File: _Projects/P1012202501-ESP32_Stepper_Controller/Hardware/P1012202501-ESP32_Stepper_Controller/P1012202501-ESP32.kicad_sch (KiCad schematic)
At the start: 6 parts, among them IC3 ESP32-WROOM-32UE-N16

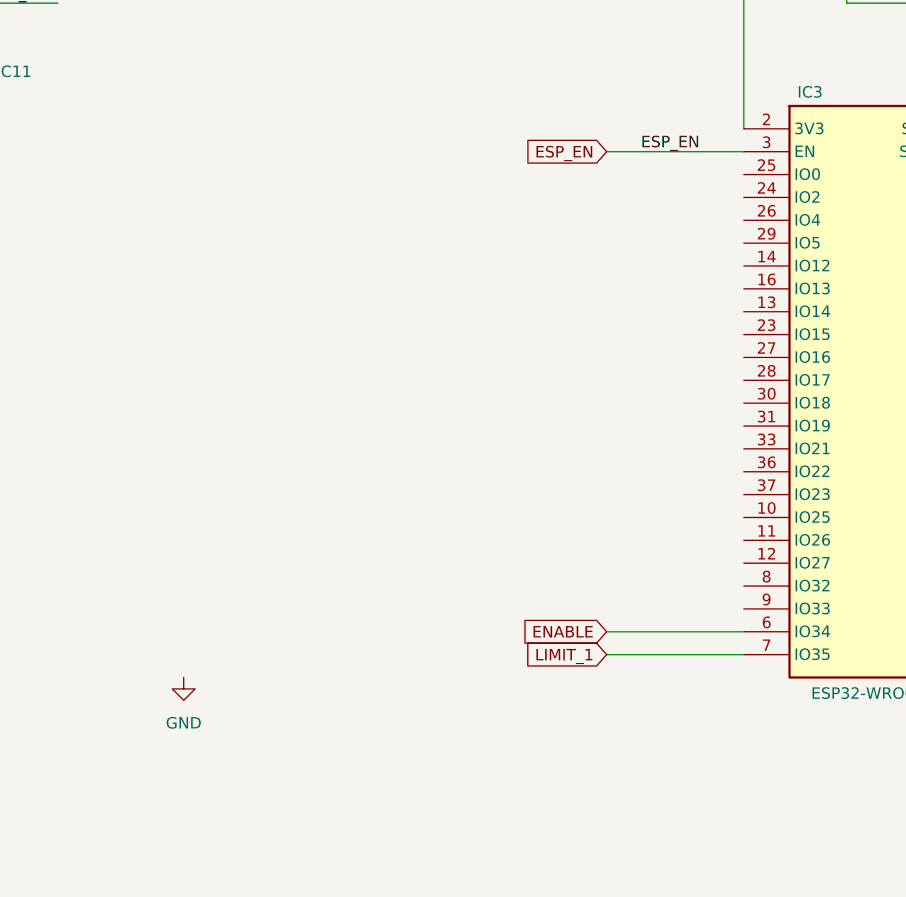
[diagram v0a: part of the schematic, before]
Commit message: Added content from latest stream.
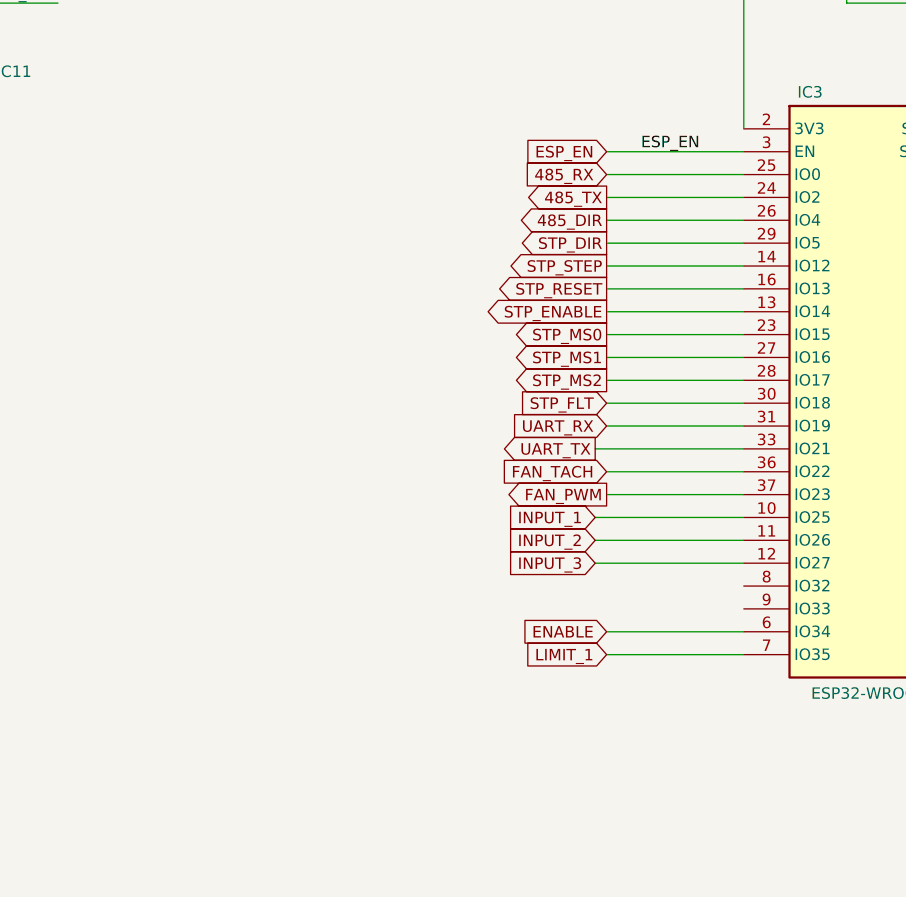
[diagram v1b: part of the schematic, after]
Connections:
- net INPUT_1: now reaches IC3.10 (IO25)
- net INPUT_2: now reaches IC3.11 (IO26)
- net INPUT_3: now reaches IC3.12 (IO27)
- net STP_ENABLE: now reaches IC3.13 (IO14)
- net STP_STEP: now reaches IC3.14 (IO12)
- net STP_RESET: now reaches IC3.16 (IO13)
- net STP_MS0: now reaches IC3.23 (IO15)
- net 485_TX: now reaches IC3.24 (IO2)
- net 485_RX: now reaches IC3.25 (IO0)
- net 485_DIR: now reaches IC3.26 (IO4)
- net STP_MS1: now reaches IC3.27 (IO16)
- net STP_MS2: now reaches IC3.28 (IO17)
- net STP_DIR: now reaches IC3.29 (IO5)
- net STP_FLT: now reaches IC3.30 (IO18)
- net UART_RX: now reaches IC3.31 (IO19)
- net UART_TX: now reaches IC3.33 (IO21)
- net FAN_TACH: now reaches IC3.36 (IO22)
- net FAN_PWM: now reaches IC3.37 (IO23)

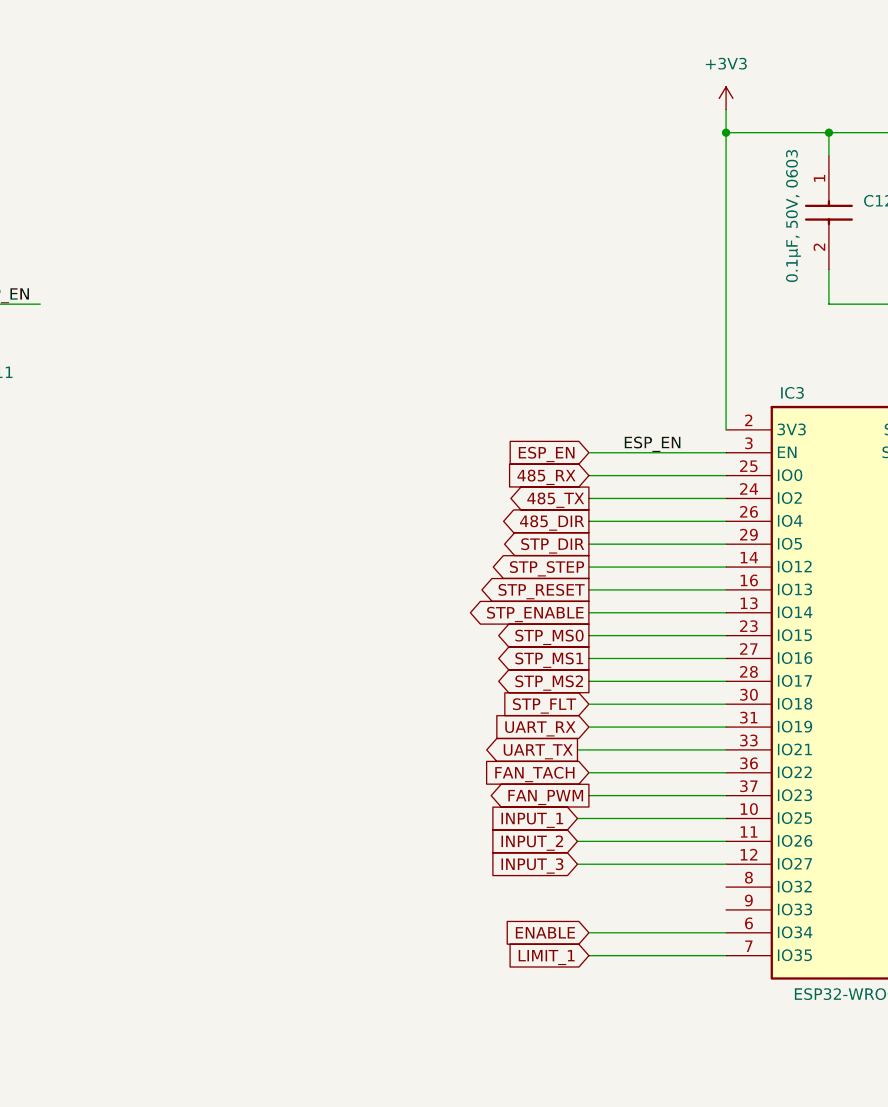
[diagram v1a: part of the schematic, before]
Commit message: Adding new content from stream.
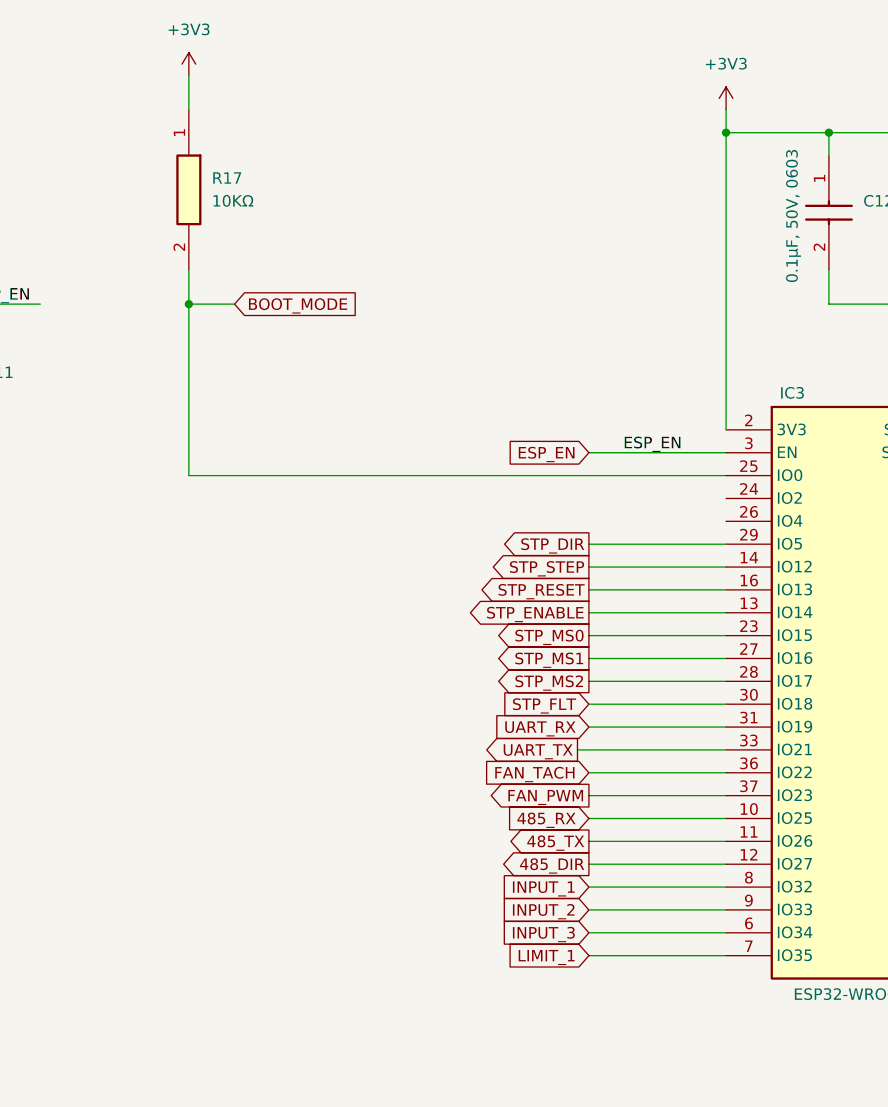
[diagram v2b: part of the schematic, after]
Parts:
- added R17: RC060310K2075AAA, COMPONENTS:RES-0603, symbol COMPONENTS:RC060310K2075AAA
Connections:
- net ENABLE is gone; now on net INPUT_3: IC3.6 (IO34)
- net +3V3: now also R17.1
- net 485_DIR: now also IC3.12 (IO27); no longer IC3.26 (IO4)
- net 485_RX: now also IC3.10 (IO25); no longer IC3.25 (IO0)
- net 485_TX: now also IC3.11 (IO26); no longer IC3.24 (IO2)
- net INPUT_1: now also IC3.8 (IO32); no longer IC3.10 (IO25)
- net INPUT_2: now also IC3.9 (IO33); no longer IC3.11 (IO26)
- net INPUT_3: no longer IC3.12 (IO27)
- new net BOOT_MODE: IC3.25 (IO0), R17.2
